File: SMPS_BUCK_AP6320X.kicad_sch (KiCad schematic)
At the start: 16 parts, among them J1 61300411121, U2 AP63205WU-7

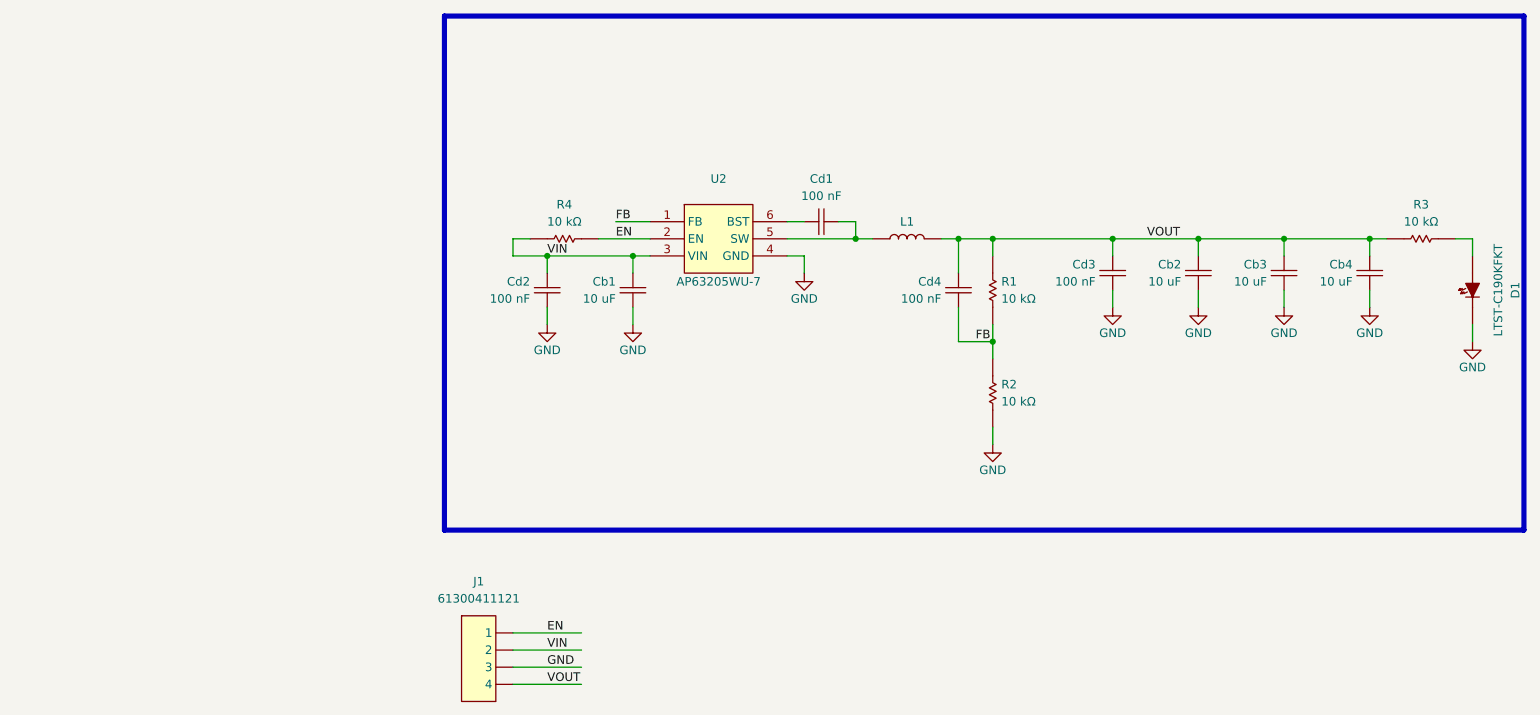
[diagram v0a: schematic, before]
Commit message: New layout.
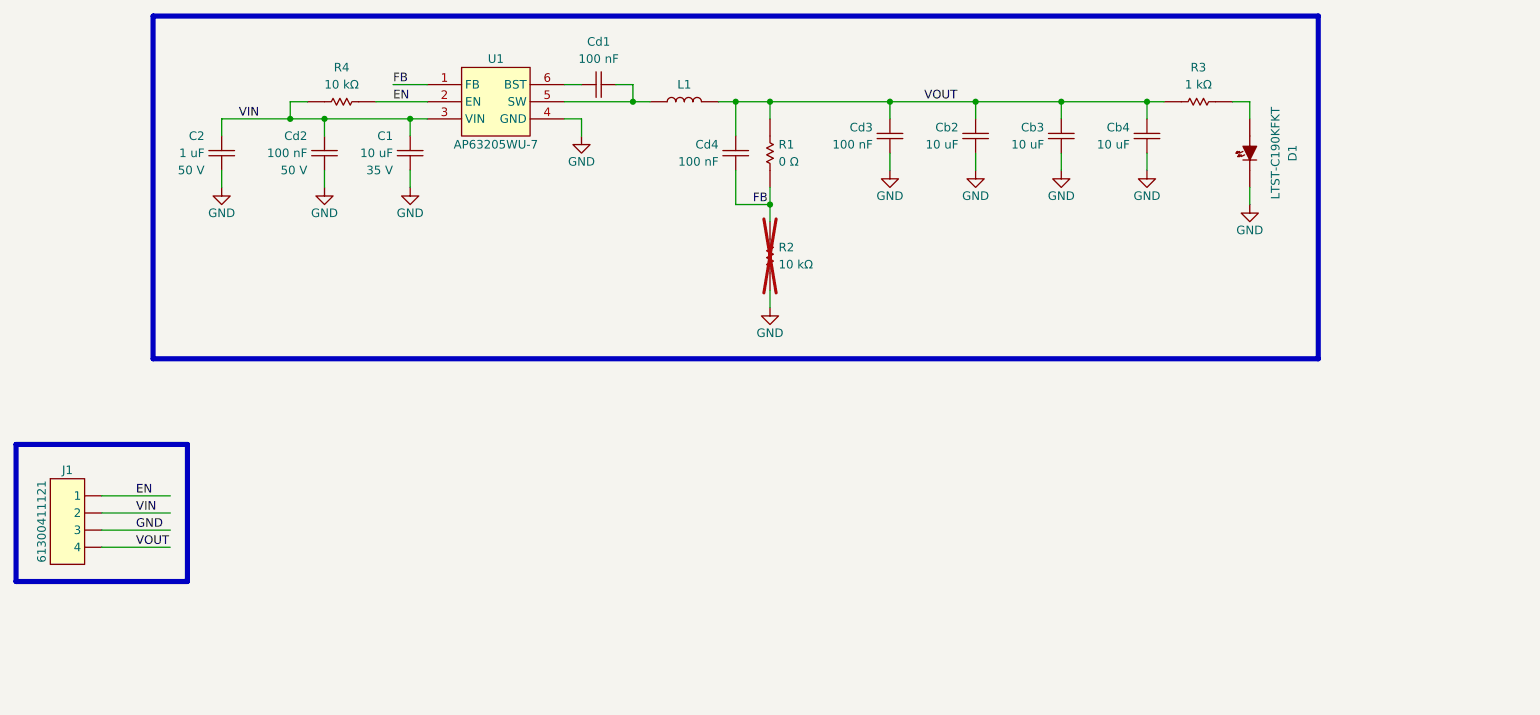
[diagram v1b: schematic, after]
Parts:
- removed Cb1: 10 uF, kicad_lib:Samsung_Electro-Mechanics_CL10B104JB8NNNC, symbol kicad_lib:Murata_Electronics_GRM188Z71A106KA73D
- removed R1, R3: 10 kΩ, kicad_lib:YAGEO_RC0603FR-070RL, symbol kicad_lib:YAGEO_RC0603FR-0710KL
- added C1: 10 uF, kicad_lib:Samsung_Electro-Mechanics_CL10B104JB8NNNC, symbol kicad_lib:Murata_Electronics_GRM188R6YA106MA73D
- added C2: 1 uF, kicad_lib:Samsung_Electro-Mechanics_CL10B104JB8NNNC, symbol kicad_lib:Samsung_Electro-Mechanics_CL10A105KB8NNNC
- added R1: 0 Ω, kicad_lib:YAGEO_RC0603FR-070RL, symbol kicad_lib:YAGEO_RC0603FR-070RL
- added R3: 1 kΩ, kicad_lib:YAGEO_RC0603FR-070RL, symbol kicad_lib:YAGEO_RC0603FR-071KL
- R2: now not fitted
- renumbered U2 to U1
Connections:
- net FB: now also R1.1
- net GND: now also C1.1, C2.1
- net VIN: now also C1.2, C2.2
- net VOUT: now also R1.2, R3.1
- net at D1.A: now also R3.2
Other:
- moved on the sheet: Cb2, Cb3, Cb4, Cd1, Cd2, Cd3, Cd4, D1, J1, L1, R4, U1
